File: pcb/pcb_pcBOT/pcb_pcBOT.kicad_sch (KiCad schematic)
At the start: 0 parts

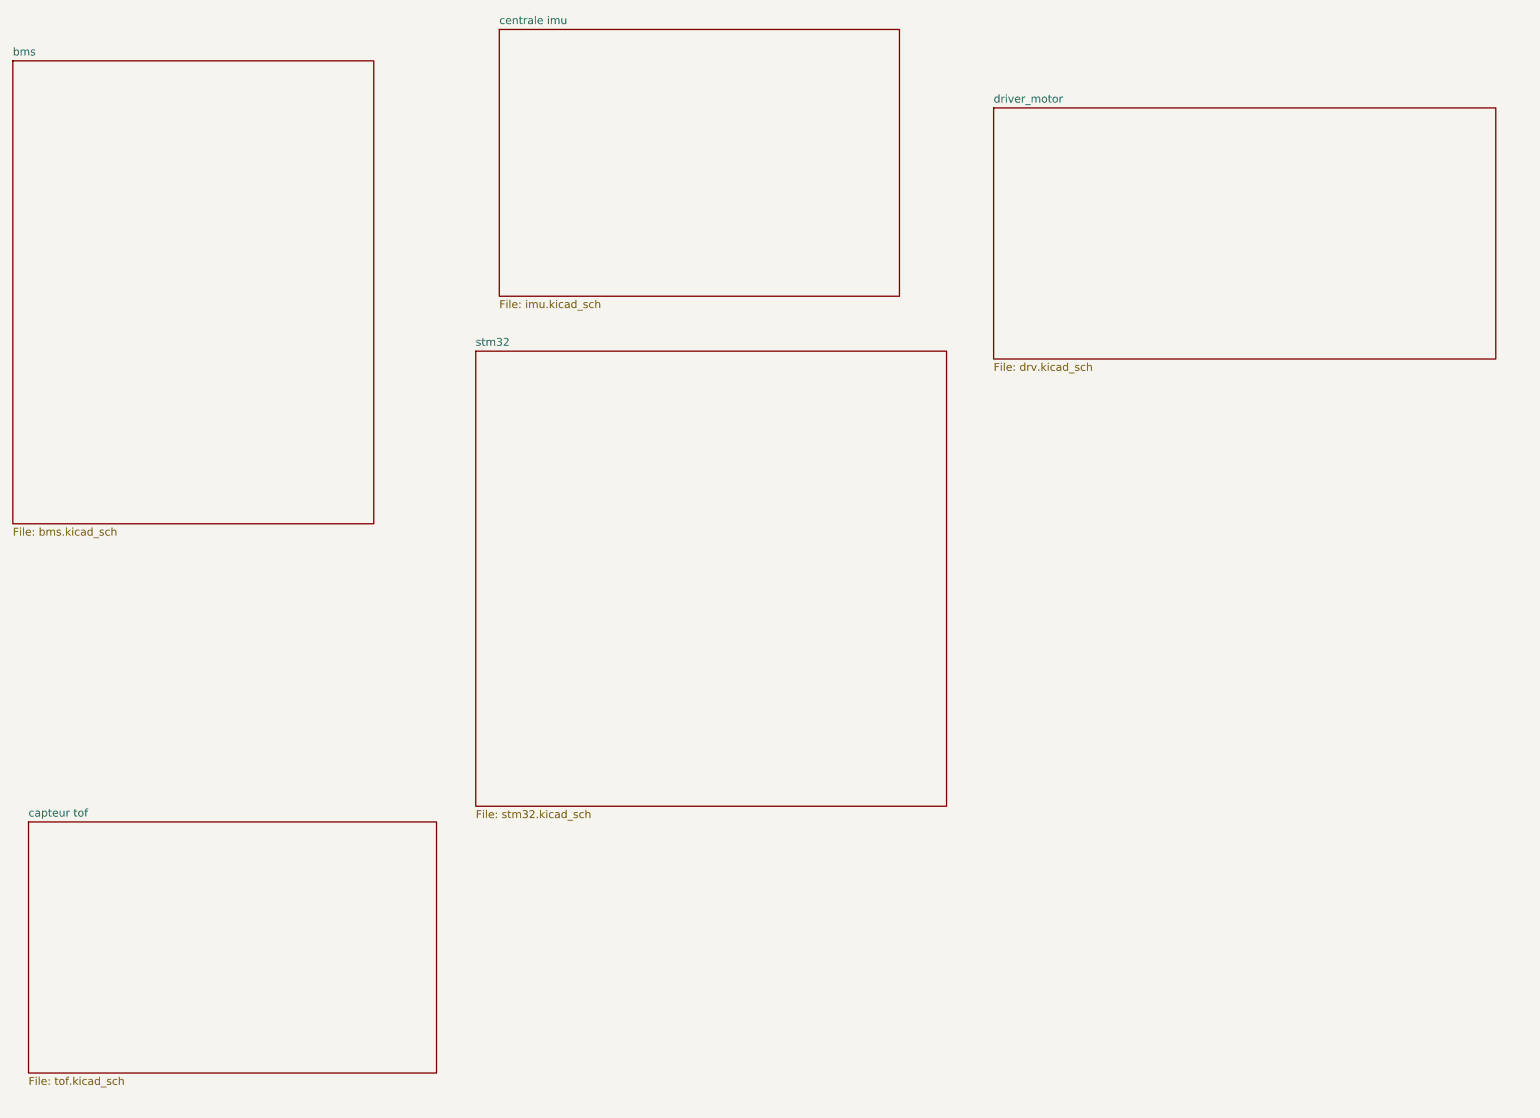
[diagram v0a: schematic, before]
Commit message: pcb
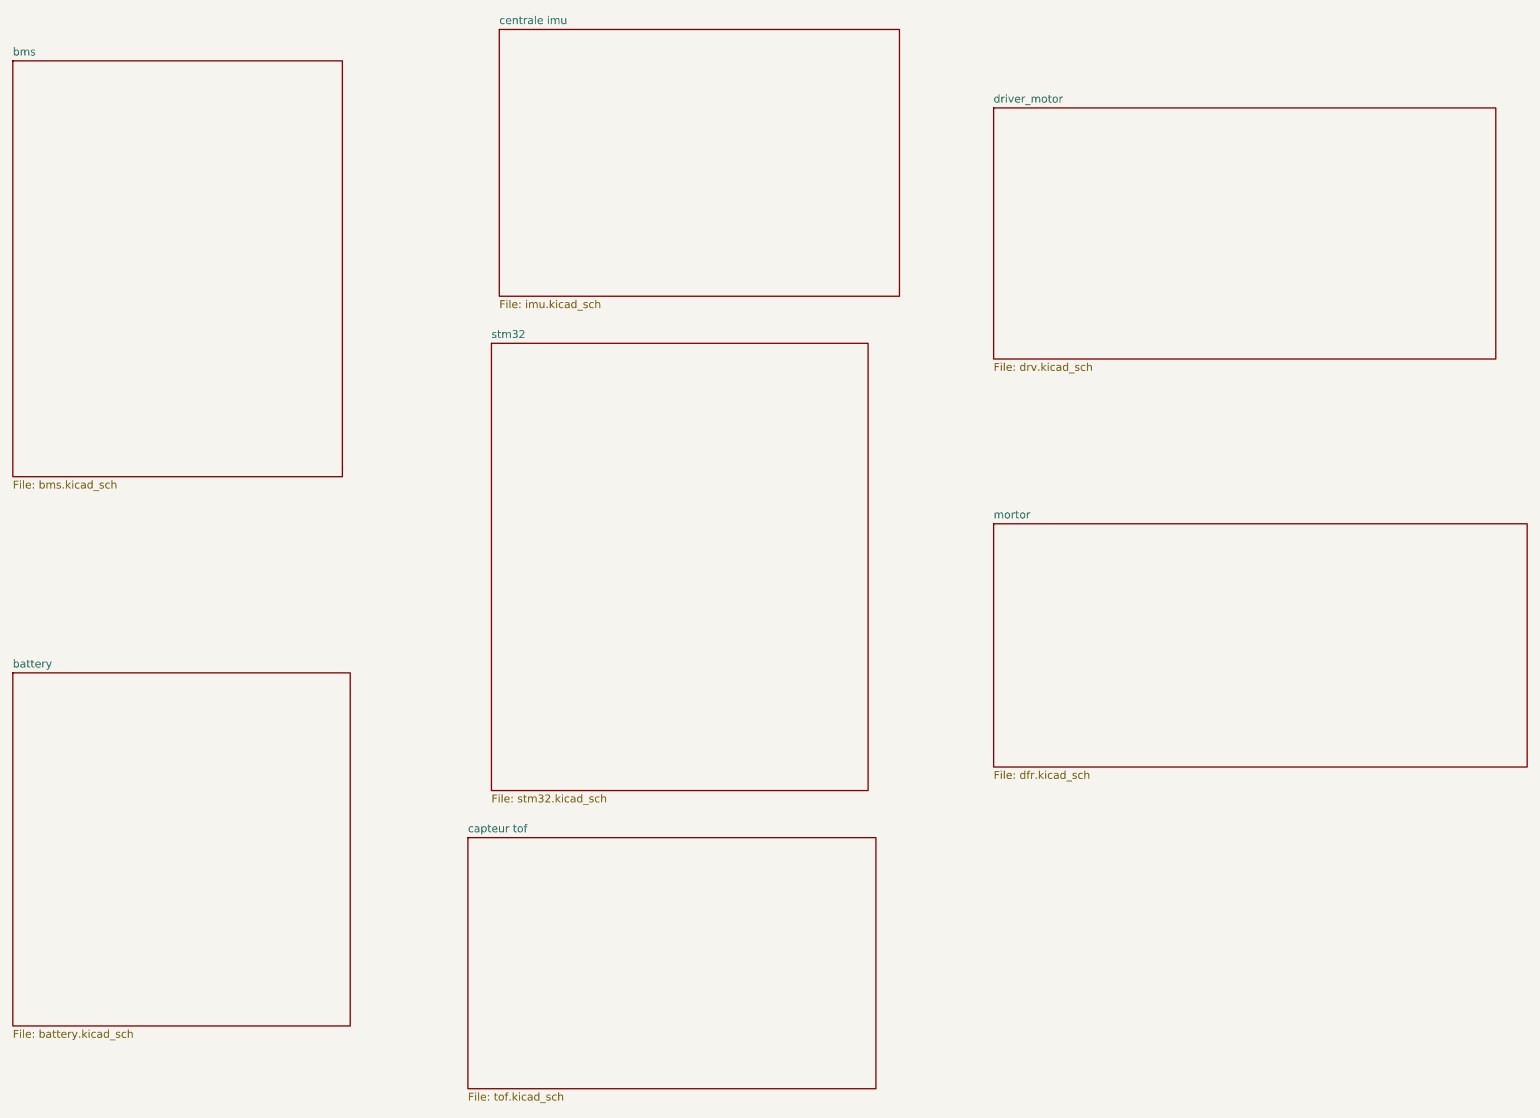
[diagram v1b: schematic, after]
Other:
- added sheet battery (battery.kicad_sch)
- added sheet mortor (dfr.kicad_sch)
- title: schematic_PcBot_2026 -> (none)
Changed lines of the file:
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@@
 (kicad_sch (version 20230121) (generator eeschema)
   (paper "A4")
-  (title_block
-    (title "schematic_PcBot_2026")
-    (rev "1.0")
-  )
-  (sheet (at 30.48 148.59) (size 66.04 40.64) (fields_autoplaced)
+  (sheet (at 27.94 124.46) (size 54.61 57.15) (fields_autoplaced)
     (stroke (width 0.1524) (type solid))
     (fill (color 0 0 0 0.0000))
-    (property "Sheetname" "capteur tof" (at 30.48 147.8784 0)
+    (property "Sheetname" "battery" (at 27.94 123.7484 0)
       (effects (font (size 1.27 1.27)) (justify left bottom))
     )
-    (property "Sheetfile" "tof.kicad_sch" (at 30.48 189.8146 0)
+    (property "Sheetfile" "battery.kicad_sch" (at 27.94 182.1946 0)
+      (effects (font (size 1.27 1.27)) (justify left top))
+    )
+    (instances
+      (project "pcb_pcBOT"
+        (path "/704e4da3-8ee7-458f-8a0f-3fc97e8dc2a6" (page "4"))
+      )
+    )
+  )
+  (sheet (at 101.6 151.13) (size 66.04 40.64) (fields_autoplaced)
+    (stroke (width 0.1524) (type solid))
+    (fill (color 0 0 0 0.0000))
+    (property "Sheetname" "capteur tof" (at 101.6 150.4184 0)
+      (effects (font (size 1.27 1.27)) (justify left bottom))
+    )
+    (property "Sheetfile" "tof.kicad_sch" (at 101.6 192.3546 0)
       (effects (font (size 1.27 1.27)) (justify left top))
     )
@@
       (project "pcb_pcBOT"
         (path "/704e4da3-8ee7-458f-8a0f-3fc97e8dc2a6" (page "5"))
+      )
+    )
+  )
+  (sheet (at 186.69 100.33) (size 86.36 39.37) (fields_autoplaced)
+    (stroke (width 0.1524) (type solid))
+    (fill (color 0 0 0 0.0000))
+    (property "Sheetname" "mortor" (at 186.69 99.6184 0)
+      (effects (font (size 1.27 1.27)) (justify left bottom))
+    )
+    (property "Sheetfile" "dfr.kicad_sch" (at 186.69 140.2846 0)
+      (effects (font (size 1.27 1.27)) (justify left top))
+    )
+    (instances
+      (project "pcb_pcBOT"
+        (path "/704e4da3-8ee7-458f-8a0f-3fc97e8dc2a6" (page "8"))
       )
     )
@@
     )
   )
-  (sheet (at 102.87 72.39) (size 76.2 73.66) (fields_autoplaced)
+  (sheet (at 105.41 71.12) (size 60.96 72.39) (fields_autoplaced)
     (stroke (width 0.1524) (type solid))
     (fill (color 0 0 0 0.0000))
-    (property "Sheetname" "stm32" (at 102.87 71.6784 0)
+    (property "Sheetname" "stm32" (at 105.41 70.4084 0)
       (effects (font (size 1.27 1.27)) (justify left bottom))
     )
-    (property "Sheetfile" "stm32.kicad_sch" (at 102.87 146.6346 0)
+    (property "Sheetfile" "stm32.kicad_sch" (at 105.41 144.0946 0)
       (effects (font (size 1.27 1.27)) (justify left top))
     )
@@
     )
   )
-  (sheet (at 27.94 25.4) (size 58.42 74.93) (fields_autoplaced)
+  (sheet (at 27.94 25.4) (size 53.34 67.31) (fields_autoplaced)
     (stroke (width 0.1524) (type solid))
     (fill (color 0 0 0 0.0000))
@@
       (effects (font (size 1.27 1.27)) (justify left bottom))
     )
-    (property "Sheetfile" "bms.kicad_sch" (at 27.94 100.9146 0)
+    (property "Sheetfile" "bms.kicad_sch" (at 27.94 93.2946 0)
       (effects (font (size 1.27 1.27)) (justify left top))
     )
